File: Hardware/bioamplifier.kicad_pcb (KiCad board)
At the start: 4 copper layers, 73.2 x 45 mm, 86 parts, among them IC1 MCP1754ST-3302E_DB, J1 Conn_01x07_Socket, J2 Conn_01x26_Pin, J3 Conn_01x07_Socket, U1 ADS1299IPAG, U10 TPD4E1B06DCKR, U11 LM2665M6, U12 TLV77333PDQNR, U2 TPD4E1B06DCKR, U3 TPD4E1B06DCKR, U4 TPD4E1B06DCKR, U5 TPD4E1B06DCKR, U6 TPS73133DBV, U7 TPS72325DBV, U8 TLV70310DBVR, U9 TPD4E1B06DCKR

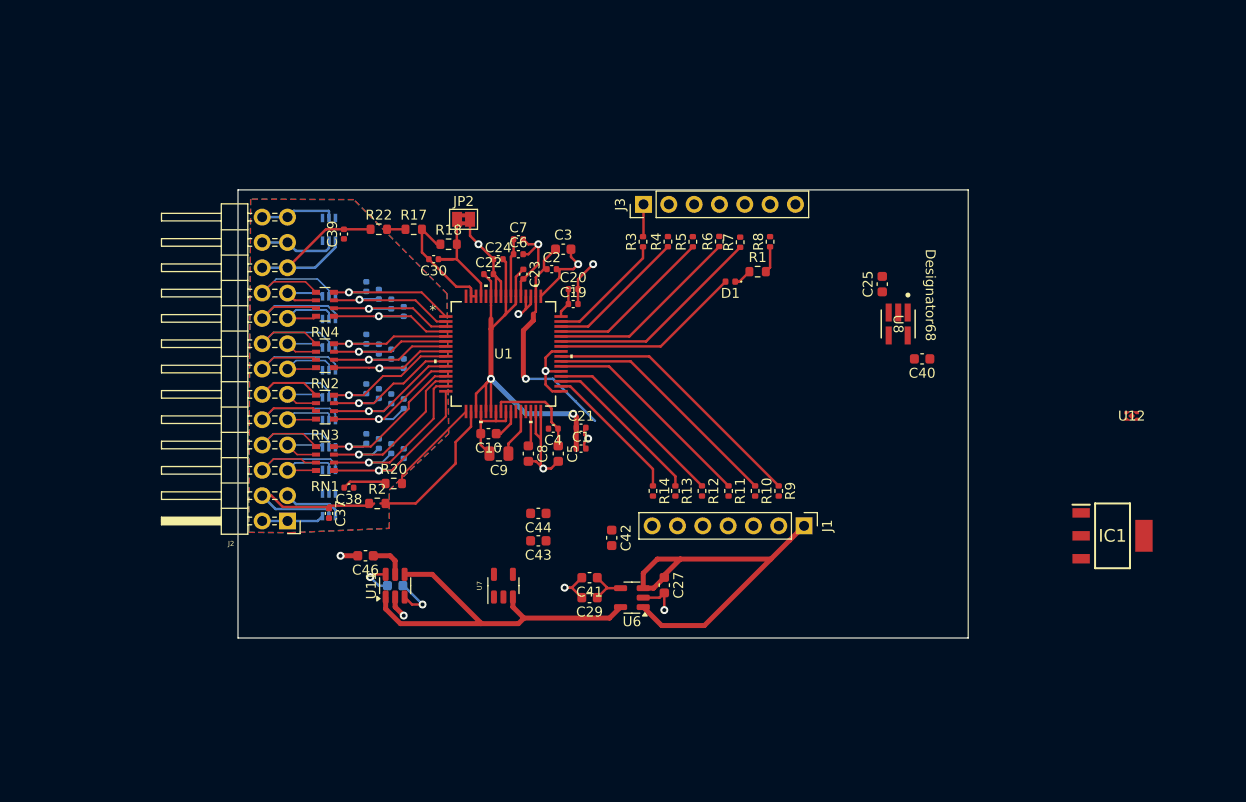
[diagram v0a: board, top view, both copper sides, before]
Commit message: Fix Last DRC Errors
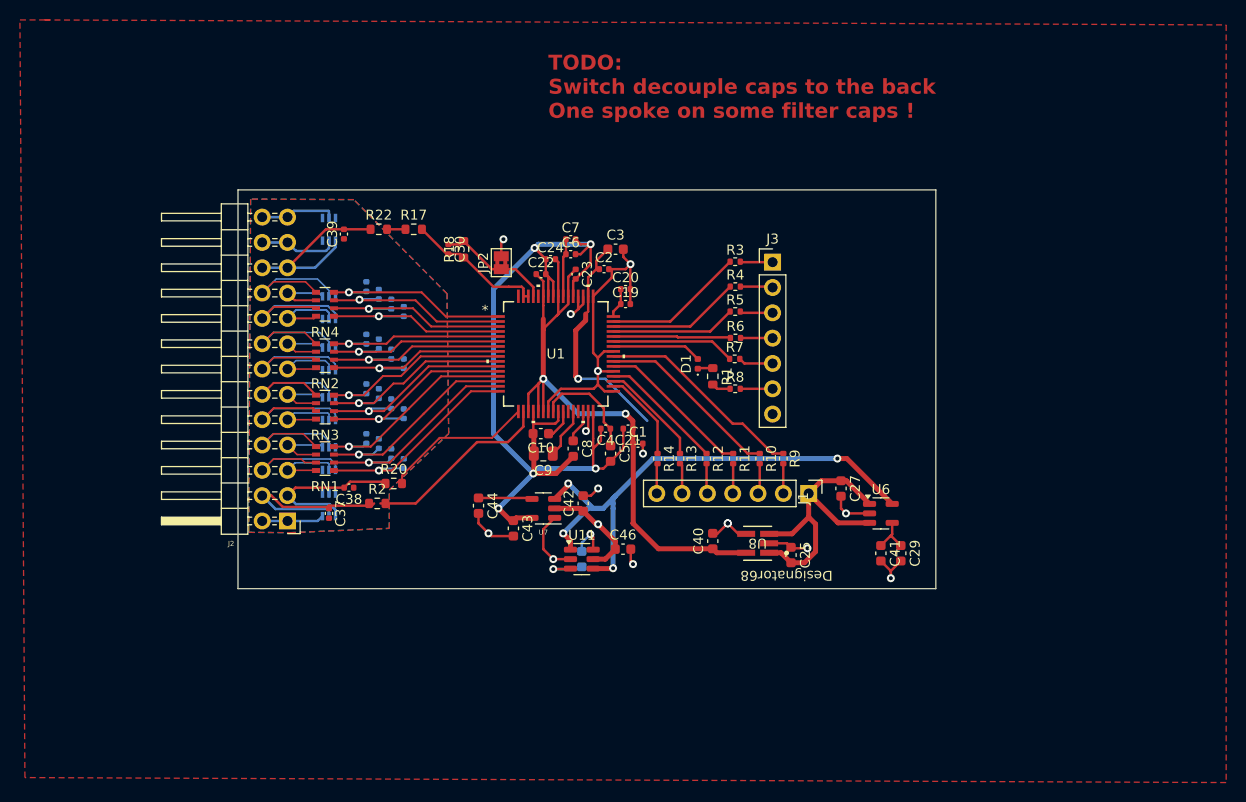
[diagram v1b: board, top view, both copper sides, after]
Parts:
- removed IC1: MCP1754ST-3302E_DB, mcp1754:SOT230P700X180-4N
- removed U12: TLV77333PDQNR, tlv77333:X2SON_DQN4_TEX
- moved C29 31.5 mm to (118.9, 108.5), turned to -90 degrees
- moved C41 29.3 mm to (116.9, 108.5), turned to -90 degrees
- moved C25 28.7 mm to (107.8, 108.7), turned to -90 degrees
- moved C40 27.8 mm to (100.0, 107.3), turned to 90 degrees
- moved U6 26.4 mm to (116.9, 104.5), turned to 0 degrees
- moved U8 26.1 mm to (104.5, 107.5), turned to 180 degrees
- moved C46 25.8 mm to (91.0, 108.1), turned to 0 degrees
- moved C27 20.2 mm to (112.9, 102.0)
- moved C45 18.9 mm to (86.9, 109.1), turned to -90 degrees
- moved U11 18.9 mm to (86.9, 109.1), turned to 0 degrees
- moved R8 15.2 mm to (102.2, 92.0), turned to 0 degrees
- moved J3 14.2 mm to (106.0, 79.3), turned to 0 degrees
- moved R7 11.7 mm to (102.2, 89.0), turned to 0 degrees
- moved R1 11.4 mm to (100.0, 90.8), turned to -90 degrees
- moved R6 9.82 mm to (102.3, 86.9), turned to 0 degrees
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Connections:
- C11 pad 1: AVSS -> GNDA
- C12 pad 1: AVSS -> GNDA
- C13 pad 1: AVSS -> GNDA
- C14 pad 1: AVSS -> GNDA
- C15 pad 1: AVSS -> GNDA
- C16 pad 1: AVSS -> GNDA
- C17 pad 1: AVSS -> GNDA
- C18 pad 1: AVSS -> GNDA
- C2 pad 1: /DVDD -> DVDD
- C25 pad 1: AVSS -> GNDA
- C26 pad 1: AVSS -> GNDA
- C28 pad 1: AVSS -> GNDA
- C3 pad 1: /DVDD -> DVDD
- C31 pad 1: AVSS -> GNDA
- C32 pad 1: AVSS -> GNDA
- C33 pad 1: AVSS -> GNDA
- C34 pad 1: AVSS -> GNDA
- C35 pad 1: AVSS -> GNDA
- C36 pad 1: AVSS -> GNDA
- C37 pad 2: AVSS -> GNDA
- C38 pad 1: AVSS -> GNDA
- C39 pad 1: AVSS -> GNDA
- C40 pad 2: AVSS -> GNDA
- C42 pad 2: AVSS -> GNDA
- C43 pad 2: AVSS -> GNDA
- C44 pad 2: AVSS -> GNDA
- C46 pad 2: AVSS -> GNDA
- J2 pad 1: AVSS -> GNDA
- J2 pad 2: AVSS -> GNDA
- JP2 pad 2: AVSS -> GNDA
- U1 pad 31: AVSS -> GNDA
- U1 pad 50: /DVDD -> DVDD
- U1 pad 60: AVSS -> GNDA
- U10 pad 3: AVSS -> GNDA
- U11 pad 2: AVSS -> GNDA
- U2 pad 3: AVSS -> GNDA
- U3 pad 3: AVSS -> GNDA
- U4 pad 3: AVSS -> GNDA
- U5 pad 3: AVSS -> GNDA
- U7 pad 1: AVSS -> GNDA
- U8 pad 2: AVSS -> GNDA
- U8 pad 4: AVSS -> GNDA
- U9 pad 3: AVSS -> GNDA
- U9 pad 4: AVSS -> GNDA
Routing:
- net AVSS: track 43.5 -> 93.0 mm, vias 6 -> 5
- net DVDD: track 38.4 -> 79.3 mm, vias 0 -> 5
- net GNDA: track 0.00 -> 33.5 mm, vias 0 -> 9
- net /DVDD: track 23.1 -> 0.00 mm, vias 1 -> 0
- net AVDD: track 47.9 -> 68.2 mm
- net GNDD: track 31.2 -> 44.9 mm
- net (no net): track 11.4 -> 0.00 mm
- net Net-(D1-A): track 19.2 -> 9.00 mm
- net 3.3V_UNREG: track 41.0 -> 31.2 mm
- net /DOUT: track 21.9 -> 12.4 mm
- net /GPIO2: track 19.6 -> 11.8 mm
- net -2.5V_UNREG: track 4.09 -> 10.9 mm, vias 0 -> 1
- net /RESET: track 18.7 -> 12.6 mm
- net /CHIP_SEL: track 24.6 -> 18.5 mm
- net /START_CONV: track 21.8 -> 15.6 mm
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- added copper zone on In2.Cu, net DVDD
- added copper zone on B.Cu, net GNDA
- added copper zone on F.Cu, net GNDA
- added copper zone on In2.Cu, net GNDA
- removed copper zone on In2.Cu, net /DVDD
- removed copper zone on B.Cu, net AVSS
- removed copper zone on F.Cu, net AVSS
- removed copper zone on In1.Cu, net AVSS
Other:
- board size 73.2 x 45 mm -> 70 x 40 mm
- board text added: "TODO: Switch decouple caps to the back One spoke on some filter caps !"
